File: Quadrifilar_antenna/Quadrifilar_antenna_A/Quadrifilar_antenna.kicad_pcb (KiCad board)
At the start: 2 copper layers, 7 parts

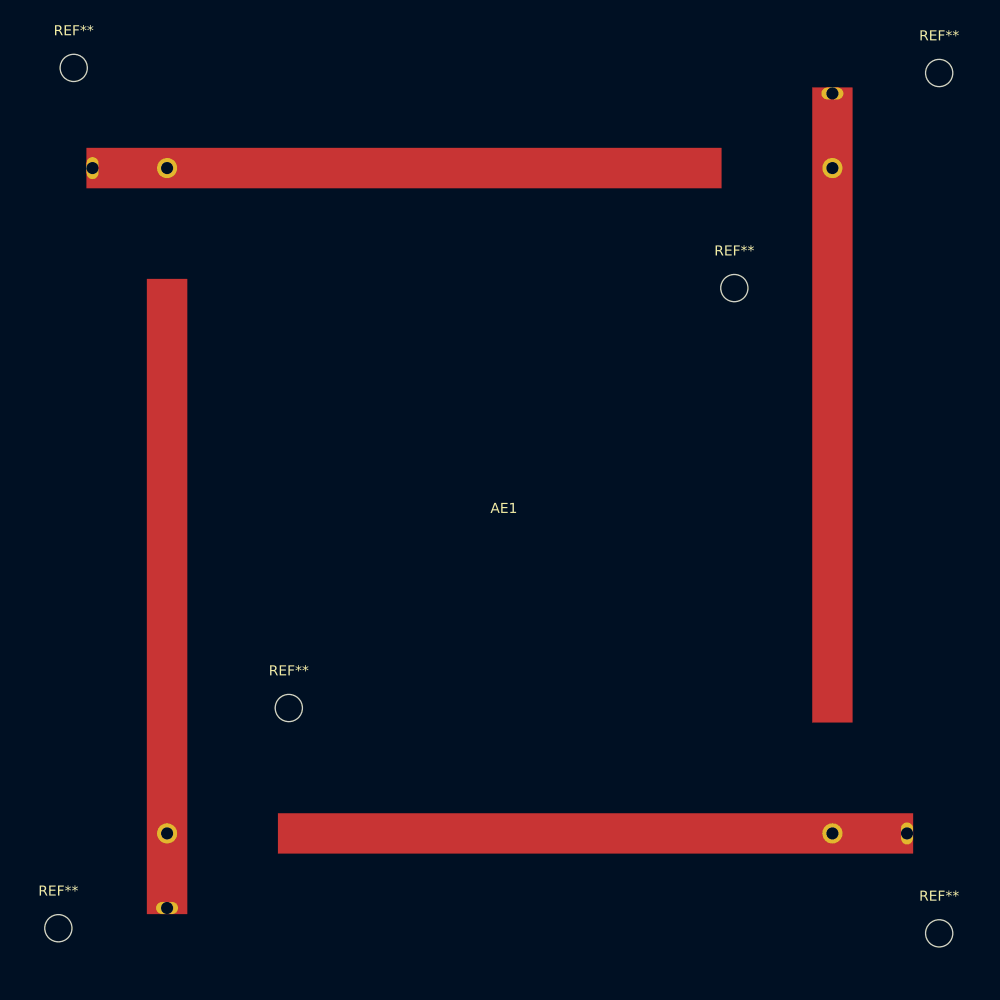
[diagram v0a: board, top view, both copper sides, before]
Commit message: update quadrifilar_antenna boards A and B
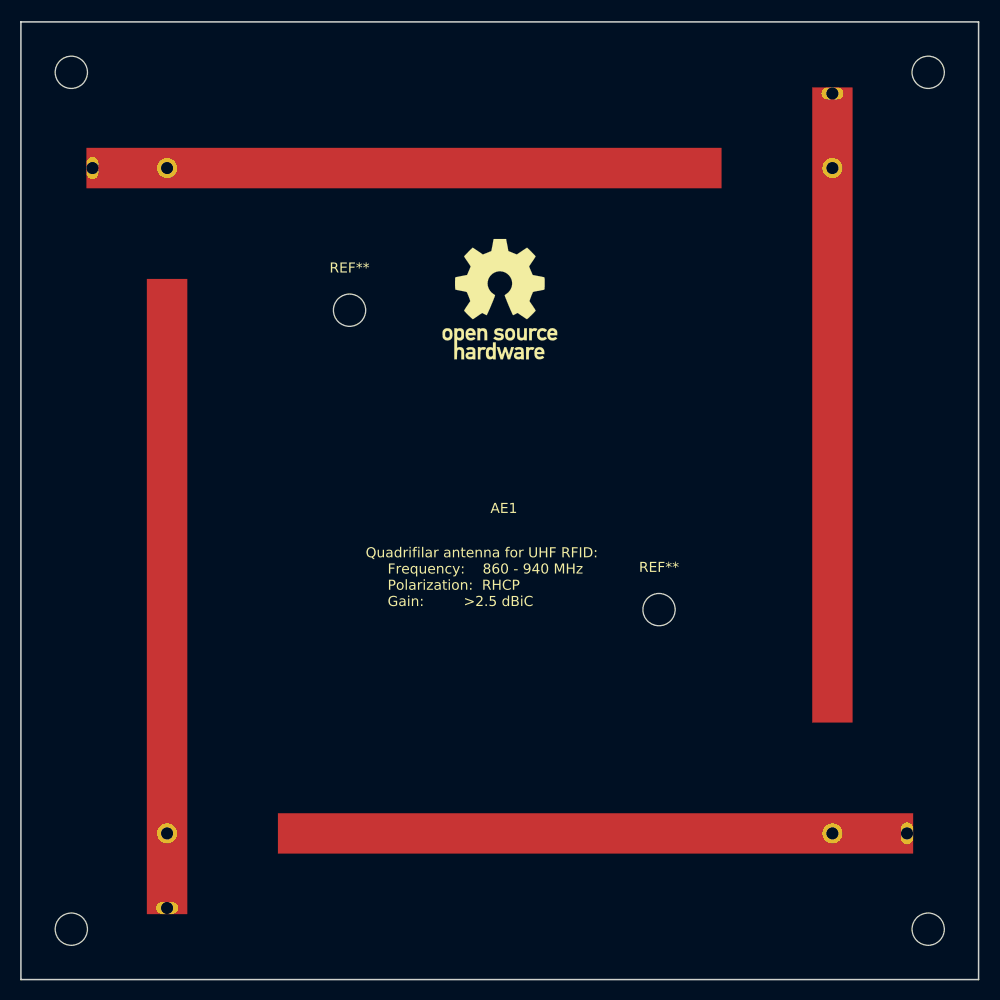
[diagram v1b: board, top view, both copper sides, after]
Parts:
- removed the REF** at (146.8, 112.3)
- removed the REF** at (191.0, 70.6)
- removed the REF** at (211.3, 134.6)
- removed the REF** at (124.0, 134.1)
- removed the REF** at (211.3, 49.3)
- removed the REF** at (125.5, 48.8)
- added  : MountingHole_3.2mm_M3, MountingHole:MountingHole_3.2mm_M3, F.Cu at (210.2, 134.2)
- added  : MountingHole_3.2mm_M3, MountingHole:MountingHole_3.2mm_M3, F.Cu at (210.2, 49.2)
- added  : MountingHole_3.2mm_M3, MountingHole:MountingHole_3.2mm_M3, F.Cu at (125.2, 49.2)
- added  : MountingHole_3.2mm_M3, MountingHole:MountingHole_3.2mm_M3, F.Cu at (125.2, 134.2)
- added REF**: MountingHole_3.2mm_M3, MountingHole:MountingHole_3.2mm_M3, F.Cu at (183.5, 102.5)
- added REF**: MountingHole_3.2mm_M3, MountingHole:MountingHole_3.2mm_M3, F.Cu at (152.8, 72.8)
- added REF**: OSHW-Logo_11.4x12mm_SilkScreen, Symbol:OSHW-Logo_11.4x12mm_SilkScreen, F.Cu at (167.7, 71.7)
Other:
- board outline added: 95 x 95 mm
- board text added: "Copyright (C) Ricardo Goncalves"
- board text added: "JLCJLCJLCJLC"
- board text added: "Quadrifilar antenna for UHF RFID: Frequency: 860 - 940 MHz Polarization: RHCP Gain: >2.5 dBiC"
